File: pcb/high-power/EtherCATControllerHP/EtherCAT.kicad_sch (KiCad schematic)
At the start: 45 parts, among them U7 LAN9252I/ML, U9 24FC512-I/SN, Y2 25 MHz, 20ppm

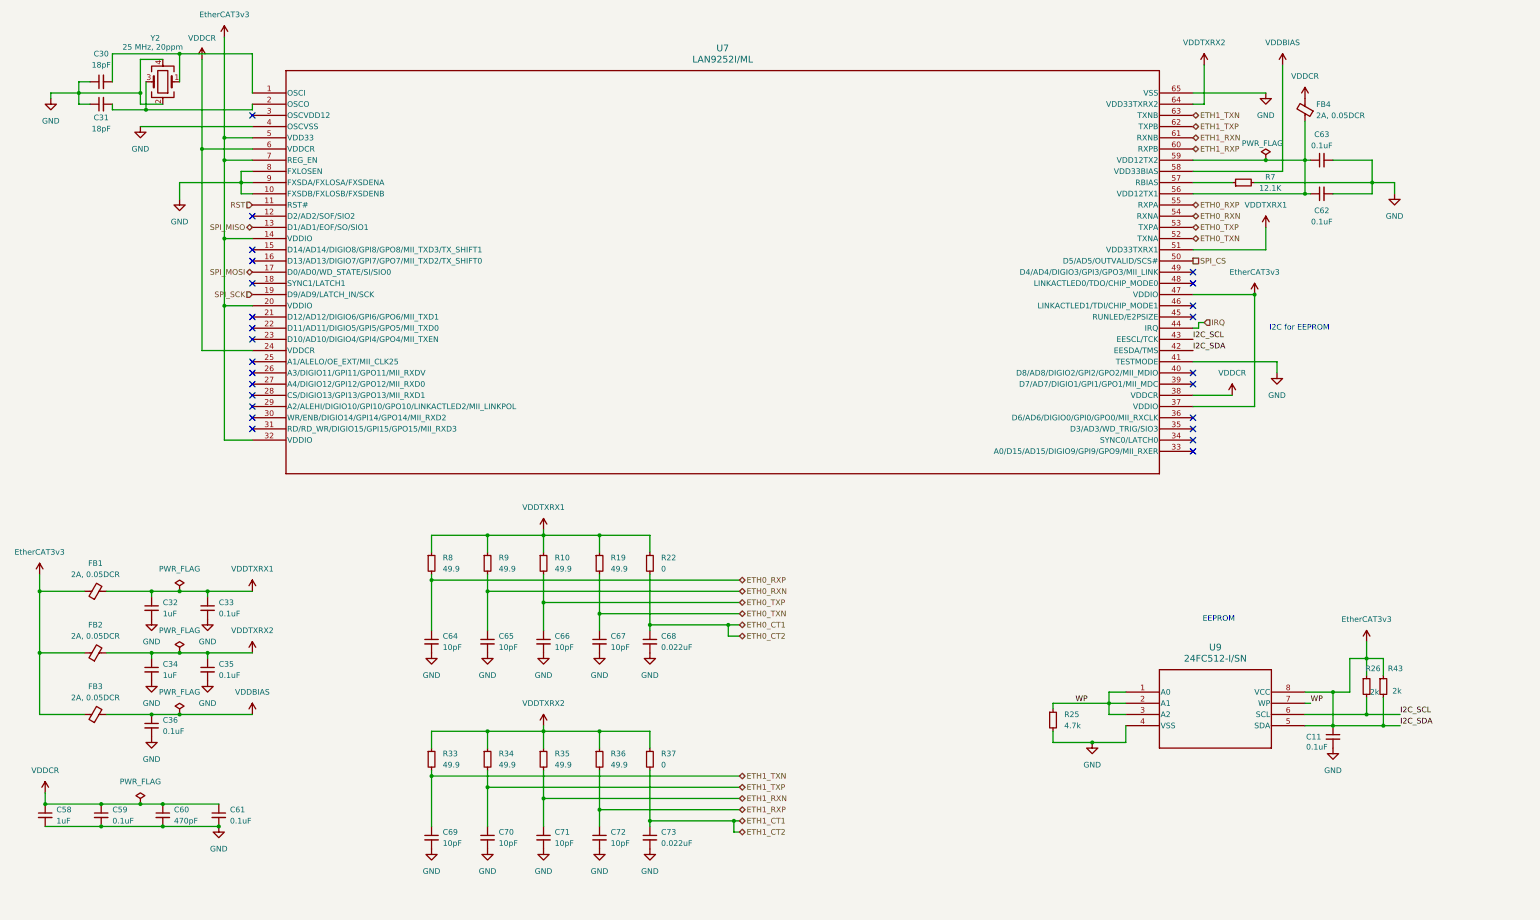
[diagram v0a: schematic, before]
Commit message: starting HP version
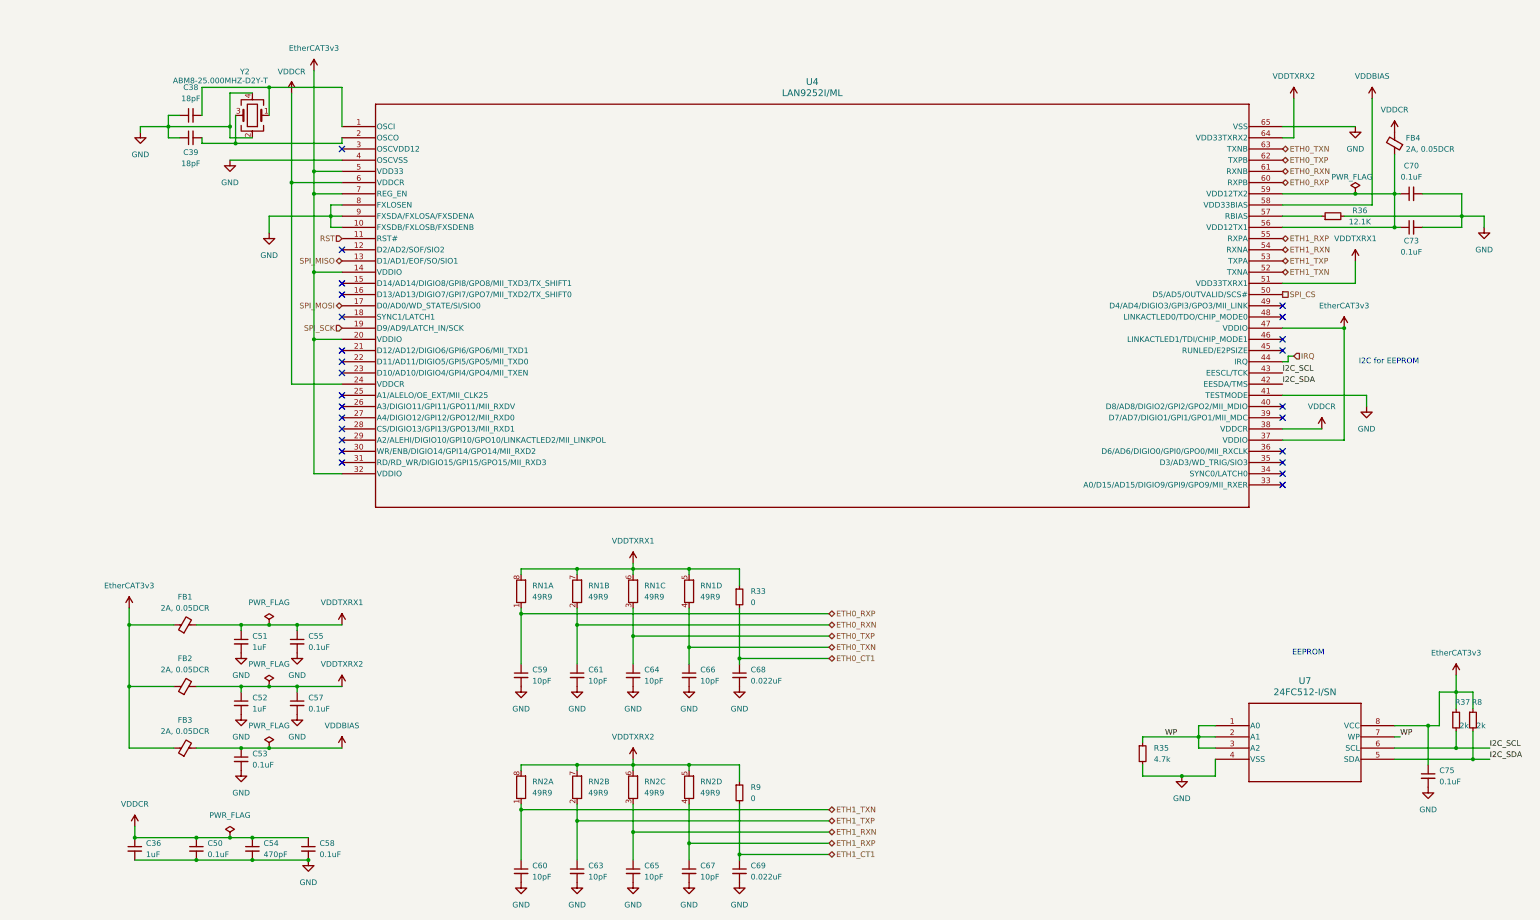
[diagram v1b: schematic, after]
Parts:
- removed C11, C33, C35, C62: 0.1uF, symbol Device:C_Small
- removed C30, C31: 18pF, symbol Device:C_Small
- removed C32, C34: 1uF, symbol Device:C_Small
- removed C71, C72: 10pF, symbol Device:C_Small
- removed R10, R19, R34: 49.9, symbol Device:R_Small
- removed R22: 0, symbol Device:R_Small
- removed R25: 4.7k, symbol Device:R_Small
- removed R26, R43: 2k, symbol Device:R_Small
- removed R7: 12.1K, symbol Device:R_Small
- removed U7: LAN9252I/ML, QFN64_ML_MCH, symbol 2024-07-01_21-03-15:LAN9252I_ML
- removed U9: 24FC512-I/SN, SOIC8_4P9X3P9MC_MCH, symbol 2024-07-03_18-39-37:24FC512-I_SN
- added C38, C39: 18pF, Capacitor_SMD:C_0402_1005Metric, symbol Device:C_Small
- added C50, C53, C55, C57, C75: 0.1uF, Capacitor_SMD:C_0603_1608Metric, symbol Device:C_Small
- added C51, C52: 1uF, Capacitor_SMD:C_0603_1608Metric, symbol Device:C_Small
- added C54: 470pF, Capacitor_SMD:C_0402_1005Metric, symbol Device:C_Small
- added RN1, RN2: 49R9, Resistor_SMD:R_Array_Convex_4x0402, symbol Device:R_Pack04_Split
- added U4: LAN9252I/ML, footprints:QFN64_ML_MCH, symbol 2024-07-01_21-03-15:LAN9252I_ML
- added U7: 24FC512-I/SN, Package_SO:SOP-8_3.9x4.9mm_P1.27mm, symbol 2024-07-03_18-39-37:24FC512-I_SN
- C36: value 0.1uF -> 1uF; footprint (none) -> Capacitor_SMD:C_0603_1608Metric; LCSC Part # (none) -> C106858
- C58: value 1uF -> 0.1uF; footprint (none) -> Capacitor_SMD:C_0603_1608Metric; LCSC Part # (none) -> C77055
- C59, C61, C63: value 0.1uF -> 10pF; footprint (none) -> Capacitor_SMD:C_0402_1005Metric; LCSC Part # (none) -> C115606
- C60: value 470pF -> 10pF; footprint (none) -> Capacitor_SMD:C_0402_1005Metric; LCSC Part # (none) -> C115606
- C64, C65, C66, C67: footprint (none) -> Capacitor_SMD:C_0402_1005Metric; LCSC Part # (none) -> C115606
- C68: footprint (none) -> Capacitor_SMD:C_0402_1005Metric; LCSC Part # (none) -> C147616
- C69: value 10pF -> 0.022uF; footprint (none) -> Capacitor_SMD:C_0402_1005Metric; LCSC Part # (none) -> C147616
- C70: value 10pF -> 0.1uF; footprint (none) -> Capacitor_SMD:C_0603_1608Metric; LCSC Part # (none) -> C77055
- C73: value 0.022uF -> 0.1uF; footprint (none) -> Capacitor_SMD:C_0603_1608Metric; LCSC Part # (none) -> C77055
- FB1, FB2, FB3, FB4: footprint (none) -> Inductor_SMD:L_1206_3216Metric; LCSC Part # (none) -> C380287
- R33, R9: value 49.9 -> 0; footprint (none) -> Resistor_SMD:R_0402_1005Metric; LCSC Part # (none) -> C106231
- R35: value 49.9 -> 4.7k; footprint (none) -> Resistor_SMD:R_0402_1005Metric; LCSC Part # (none) -> C105871
- R36: value 49.9 -> 12.1K; footprint (none) -> Resistor_SMD:R_0402_1005Metric; LCSC Part # (none) -> C281773
- R37: value 0 -> 2k; footprint (none) -> Resistor_SMD:R_0402_1005Metric; LCSC Part # (none) -> C144035
- R8: value 49.9 -> 2k; footprint (none) -> Resistor_SMD:R_0402_1005Metric; LCSC Part # (none) -> C144035
- Y2: value 25 MHz, 20ppm -> ABM8-25.000MHZ-D2Y-T; footprint (none) -> Crystal:Crystal_SMD_3225-4Pin_3.2x2.5mm; LCSC Part # (none) -> C179643; LCSC Part Number C179643 -> (none)
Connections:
- net ETH0_CT1: now also R33.2
- net ETH0_RXN: now also C61.1, RN1.2 (R2.1), U4.61 (RXNB); no longer C65.1, R9.2
- net ETH0_RXP: now also C59.1, RN1.1 (R1.1), U4.60 (RXPB); no longer C64.1, R8.2
- net ETH0_TXN: now also C66.1, RN1.4 (R4.1), U4.63 (TXNB); no longer C67.1
- net ETH0_TXP: now also C64.1, RN1.3 (R3.1), U4.62 (TXPB); no longer C66.1
- net ETH1_CT1: now also C69.1, R9.2; no longer C73.1, R37.2
- net ETH1_RXN: now also C65.1, RN2.3 (R3.1), U4.54 (RXNA); no longer R35.2
- net ETH1_RXP: now also C67.1, RN2.4 (R4.1), U4.55 (RXPA); no longer R36.2
- net ETH1_TXN: now also C60.1, RN2.1 (R1.1), U4.52 (TXNA); no longer C69.1, R33.2
- net ETH1_TXP: now also C63.1, RN2.2 (R2.1), U4.53 (TXPA); no longer C70.1
- net EtherCAT3v3: now also R37.1, R8.1, C75.1, U4.14 (VDDIO), U4.20 (VDDIO), U4.32 (VDDIO), U4.37 (VDDIO), U4.47 (VDDIO), U4.5 (VDD33), U4.7 (REG_EN), U7.8 (VCC)
- net GND: now also R35.2, R36.2, C38.1, C39.1, C50.2, C51.2, C52.2, C53.2, C54.2, C55.2, C57.2, C75.2, U4.10 (FXSDB/FXLOSB/FXSDENB), U4.4 (OSCVSS), U4.41 (TESTMODE), U4.65 (VSS), U4.8 (FXLOSEN), U4.9 (FXSDA/FXLOSA/FXSDENA), U7.4 (VSS)
- net I2C_SCL: now also R37.2, U4.43 (EESCL/TCK), U7.6 (SCL)
- net IRQ: now also U4.44 (IRQ)
- net RST: now also U4.11 (RST#)
- net SPI_CS: now also U4.50 (D5/AD5/OUTVALID/SCS#)
- net SPI_MISO: now also U4.13 (D1/AD1/EOF/SO/SIO1)
- net SPI_MOSI: now also U4.17 (D0/AD0/WD_STATE/SI/SIO0)
- net SPI_SCK: now also U4.19 (D9/AD9/LATCH_IN/SCK)
- net VDDBIAS: now also C53.1, U4.58 (VDD33BIAS); no longer C36.1
- net VDDCR: now also C36.1, C50.1, C54.1, U4.24 (VDDCR), U4.38 (VDDCR), U4.6 (VDDCR); no longer C59.1, C60.1, C61.1
- net VDDTXRX1: now also R33.1, C51.1, C55.1, RN1.5 (R4.2), RN1.6 (R3.2), RN1.7 (R2.2), RN1.8 (R1.2), U4.51 (VDD33TXRX1); no longer R8.1, R9.1
- net VDDTXRX2: now also R9.1, C52.1, C57.1, RN2.5 (R4.2), RN2.6 (R3.2), RN2.7 (R2.2), RN2.8 (R1.2), U4.64 (VDD33TXRX2); no longer R33.1, R35.1, R36.1, R37.1
- net WP: now also R35.1, U7.1 (A0), U7.2 (A1), U7.3 (A2), U7.7 (WP)
- net at Y2.1: now also C38.2, U4.1 (OSCI)
- net at Y2.3: now also C39.2, U4.2 (OSCO)
- net at FB4.1: now also C70.1, C73.1, U4.56 (VDD12TX1), U4.59 (VDD12TX2); no longer C63.1
- new net: R36.1, U4.57 (RBIAS)
- new net I2C_SDA: R8.2, U4.42 (EESDA/TMS), U7.5 (SDA)

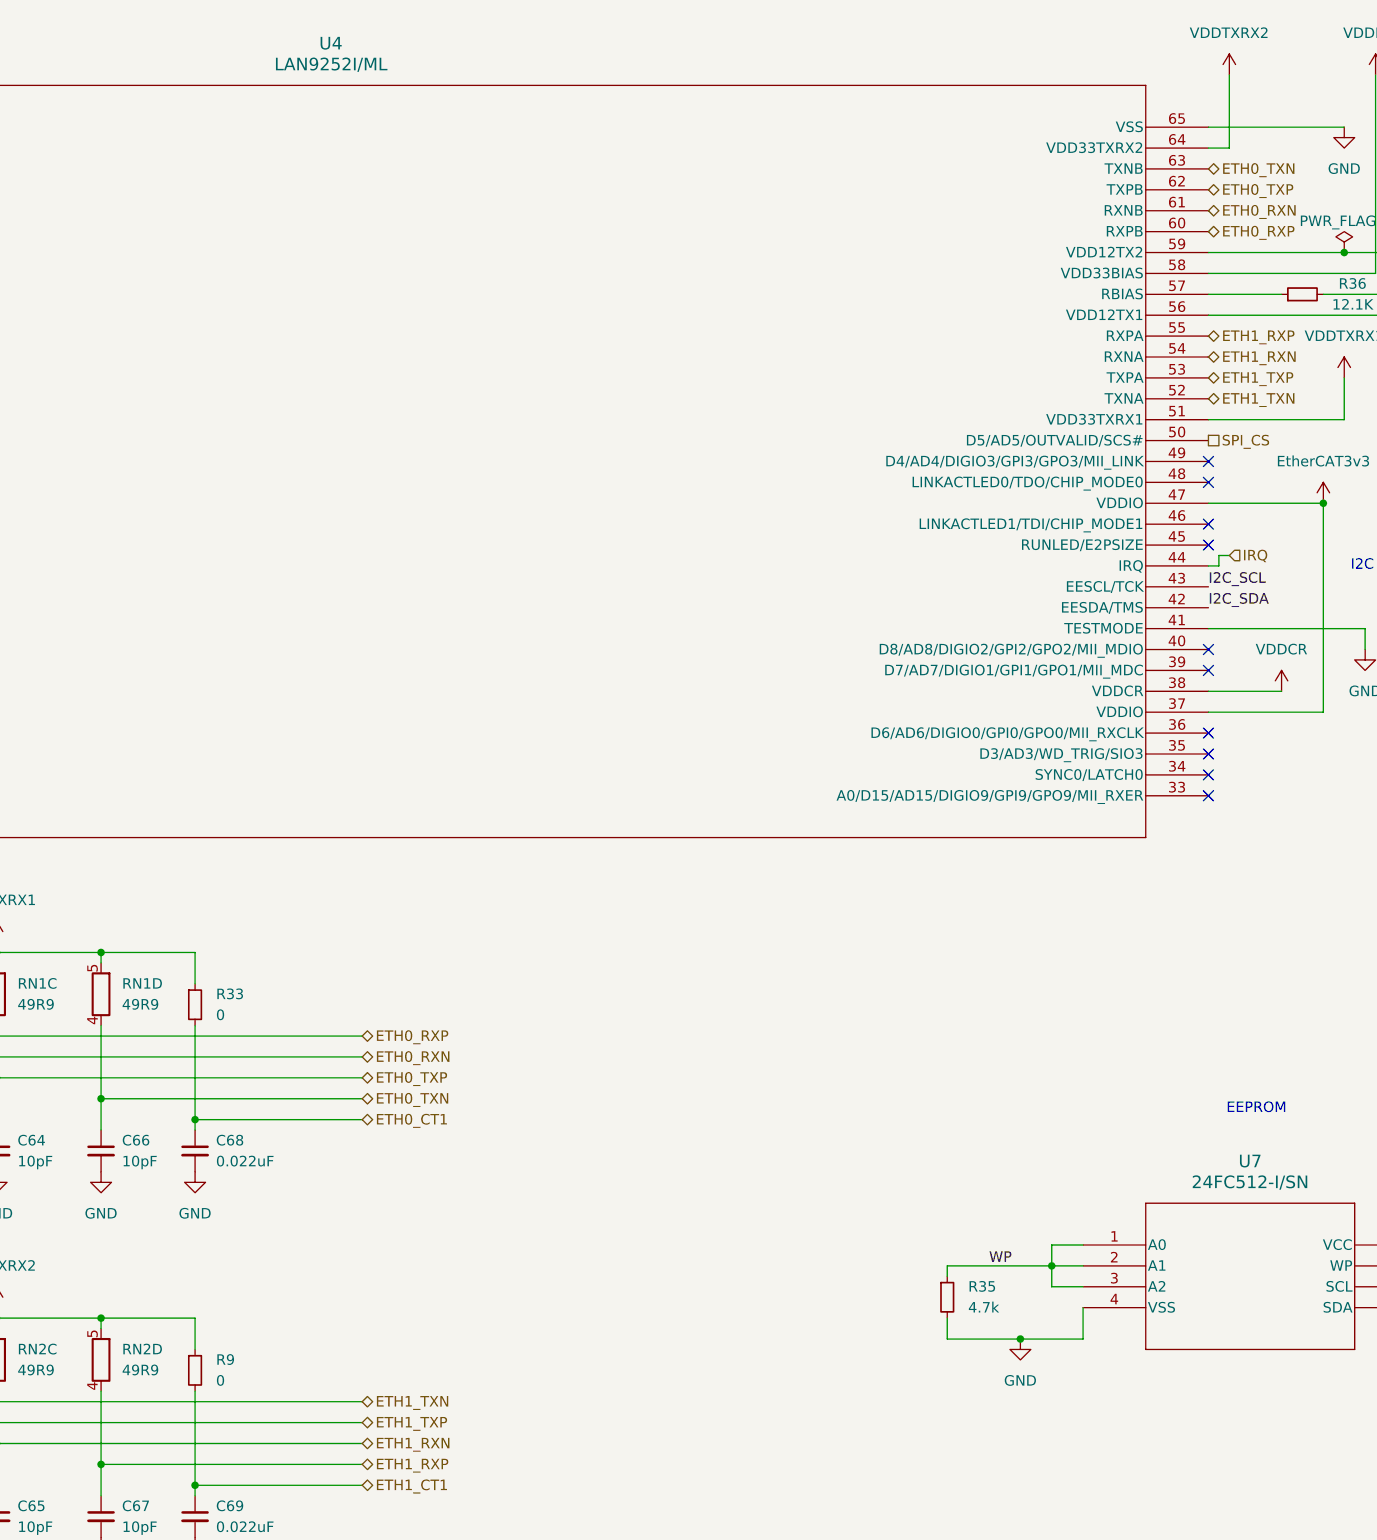
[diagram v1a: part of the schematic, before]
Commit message: stash before via stitching
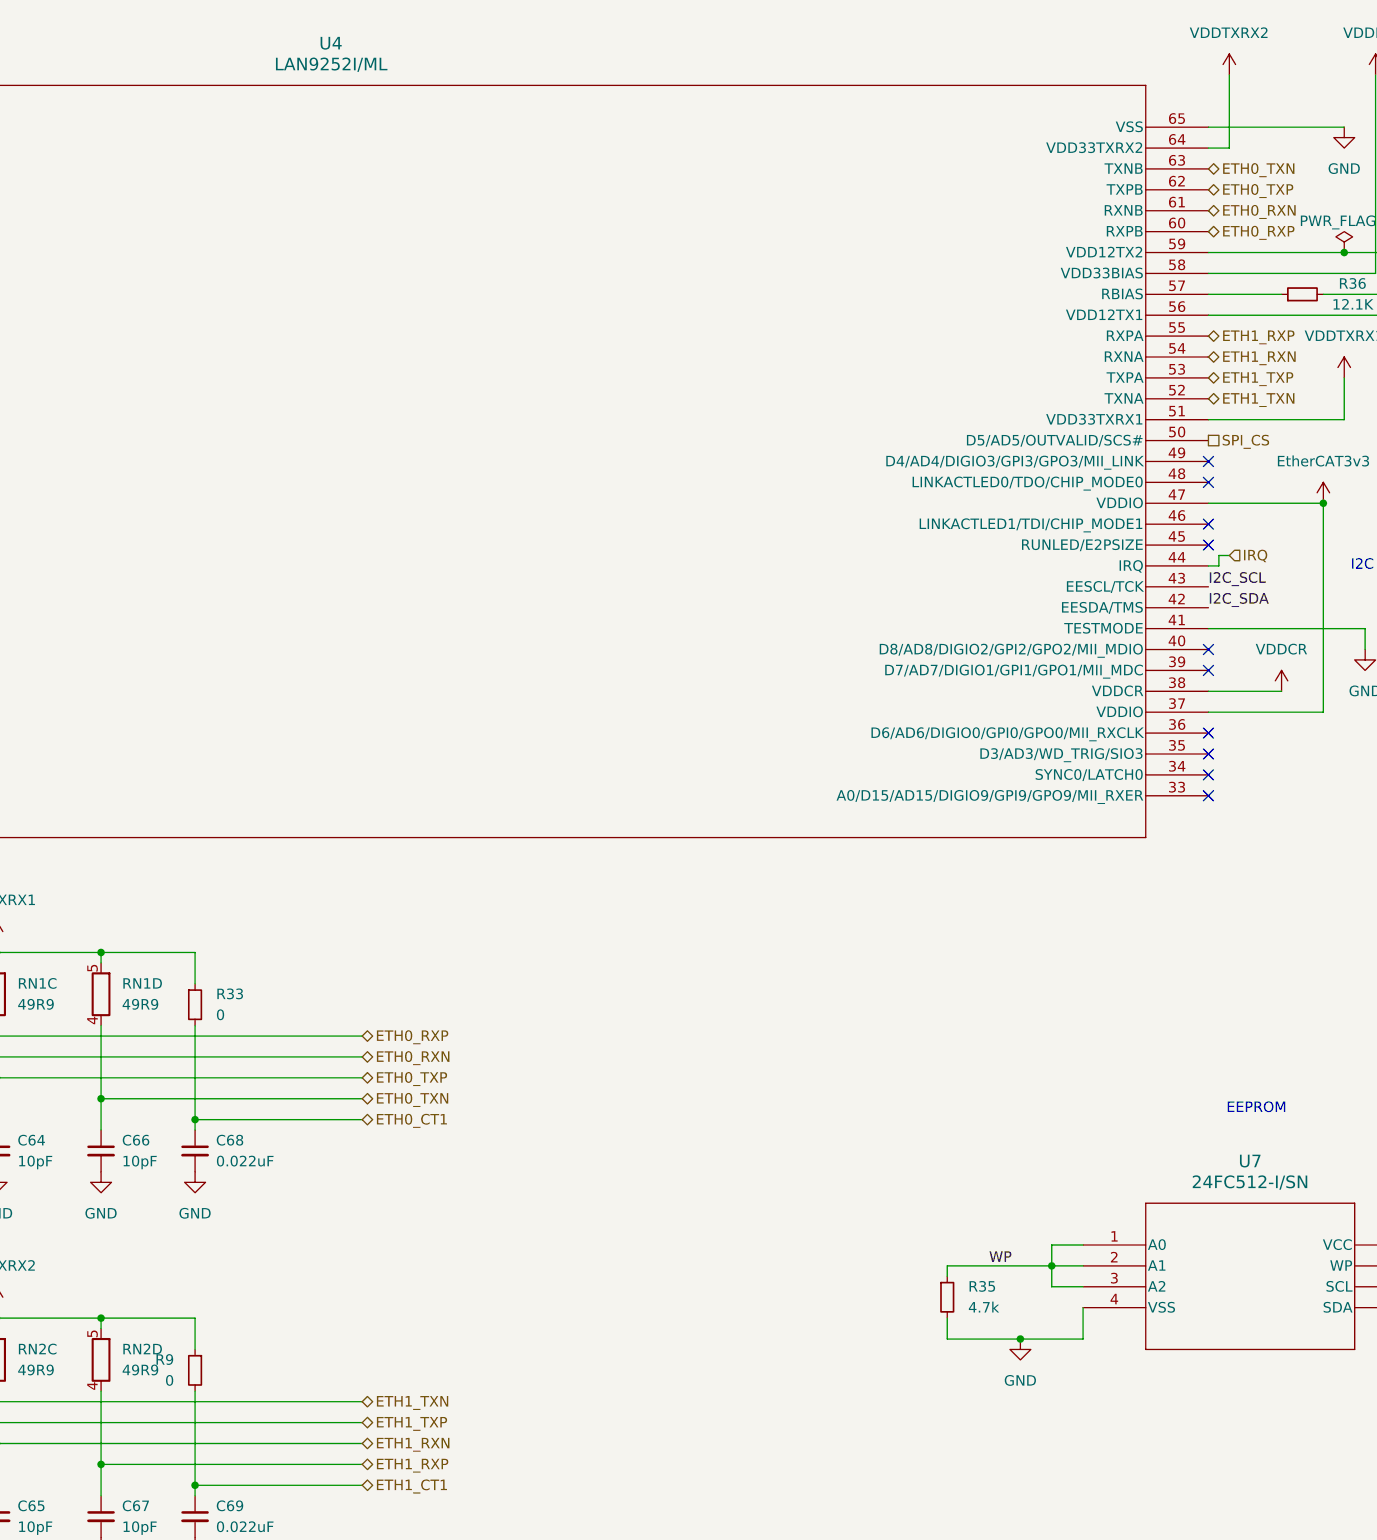
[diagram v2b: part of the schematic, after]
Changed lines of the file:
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@@
 	(wire
 		(pts
-			(xy 314.96 59.69) (xy 312.42 59.69)
-		)
-		(stroke
-			(width 0)
-			(type default)
-		)
-	)
-	(wire
-		(pts
 			(xy 165.1 172.72) (xy 165.1 179.07)
 		)
@@
 	(wire
 		(pts
+			(xy 312.42 59.69) (xy 314.96 59.69)
+		)
+		(stroke
+			(width 0)
+			(type default)
+		)
+	)
+	(wire
+		(pts
 			(xy 92.71 72.39) (xy 92.71 67.31)
 		)
@@
 		)
 	)
-	(hierarchical_label "ETH1_RXP"
+	(hierarchical_label "ETH0_TXP"
 		(shape bidirectional)
-		(at 312.42 82.55 0)
+		(at 312.42 64.77 0)
 		(fields_autoplaced yes)
 		(effects
@@
 		)
 	)
-	(hierarchical_label "ETH0_TXP"
+	(hierarchical_label "ETH0_RXP"
 		(shape bidirectional)
-		(at 312.42 64.77 0)
+		(at 312.42 69.85 0)
 		(fields_autoplaced yes)
 		(effects
@@
 		)
 	)
-	(hierarchical_label "ETH1_TXN"
+	(hierarchical_label "SPI_MISO"
 		(shape bidirectional)
-		(at 312.42 90.17 0)
+		(at 99.06 87.63 180)
+		(fields_autoplaced yes)
+		(effects
+			(font
+				(size 1.27 1.27)
+			)
+			(justify right)
+		)
+	)
+	(hierarchical_label "ETH0_TXN"
+		(shape bidirectional)
+		(at 312.42 62.23 0)
 		(fields_autoplaced yes)
 		(effects
@@
 		)
 	)
-	(hierarchical_label "SPI_MISO"
+	(hierarchical_label "ETH1_RXP"
 		(shape bidirectional)
-		(at 99.06 87.63 180)
+		(at 312.42 82.55 0)
 		(fields_autoplaced yes)
 		(effects
@@
 				(size 1.27 1.27)
 			)
-			(justify right)
+			(justify left)
 		)
 	)
-	(hierarchical_label "ETH0_CT1"
+	(hierarchical_label "ETH1_TXN"
 		(shape bidirectional)
-		(at 209.55 177.8 0)
+		(at 312.42 90.17 0)
 		(fields_autoplaced yes)
 		(effects
@@
 		)
 	)
-	(hierarchical_label "ETH1_RXN"
+	(hierarchical_label "ETH1_TXP"
 		(shape bidirectional)
-		(at 209.55 217.17 0)
+		(at 312.42 87.63 0)
 		(fields_autoplaced yes)
 		(effects
@@
 		)
 	)
-	(hierarchical_label "IRQ"
-		(shape input)
-		(at 314.96 109.22 0)
+	(hierarchical_label "ETH0_CT1"
+		(shape bidirectional)
+		(at 209.55 177.8 0)
 		(fields_autoplaced yes)
 		(effects
@@
 		)
 	)
-	(hierarchical_label "ETH0_TXN"
+	(hierarchical_label "ETH1_RXN"
 		(shape bidirectional)
-		(at 312.42 62.23 0)
+		(at 209.55 217.17 0)
+		(fields_autoplaced yes)
+		(effects
+			(font
+				(size 1.27 1.27)
+			)
+			(justify left)
+		)
+	)
+	(hierarchical_label "IRQ"
+		(shape input)
+		(at 314.96 109.22 0)
 		(fields_autoplaced yes)
 		(effects
@@
 		)
 	)
-	(hierarchical_label "ETH1_TXP"
-		(shape bidirectional)
-		(at 312.42 87.63 0)
-		(fields_autoplaced yes)
-		(effects
-			(font
-				(size 1.27 1.27)
-			)
-			(justify left)
-		)
-	)
-	(hierarchical_label "ETH0_RXP"
-		(shape bidirectional)
-		(at 312.42 69.85 0)
-		(fields_autoplaced yes)
-		(effects
-			(font
-				(size 1.27 1.27)
-			)
-			(justify left)
-		)
-	)
 	(hierarchical_label "SPI_SCK"
 		(shape input)
@@
 		(lib_id "Device:R_Small")
 		(at 189.23 208.28 0)
+		(mirror y)
 		(unit 1)
 		(exclude_from_sim no)
@@
 		(on_board yes)
 		(dnp no)
-		(fields_autoplaced yes)
 		(property "Reference" "R9"
-			(at 191.77 207.0099 0)
+			(at 186.69 207.0099 0)
 			(effects
 				(font
@@
 		)
 		(property "Value" "0"
-			(at 191.77 209.5499 0)
+			(at 186.69 209.5499 0)
 			(effects
 				(font
